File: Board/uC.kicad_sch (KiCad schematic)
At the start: 27 parts, among them U3 MP6612, U4 STM32F030K6Tx

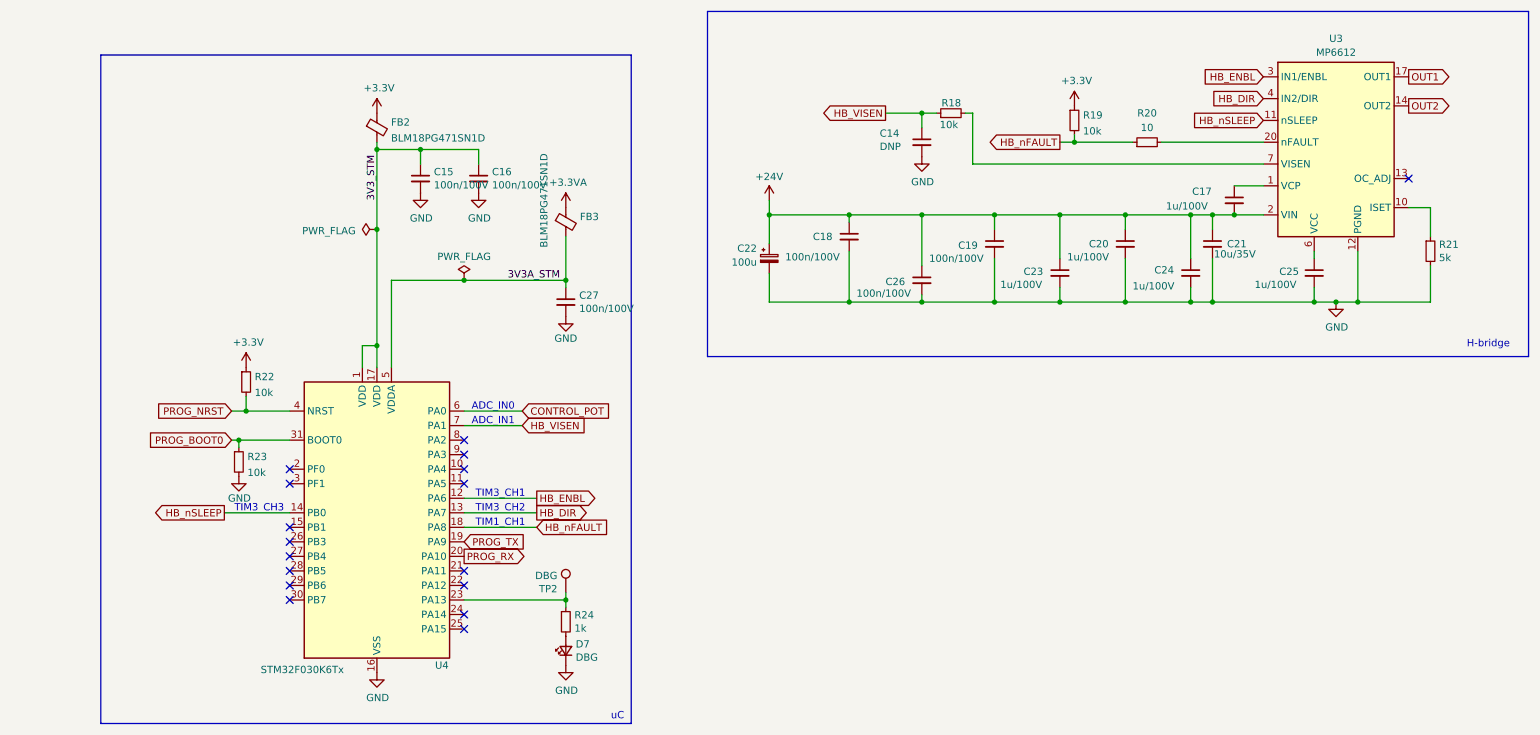
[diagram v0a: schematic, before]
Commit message: WIP on routing
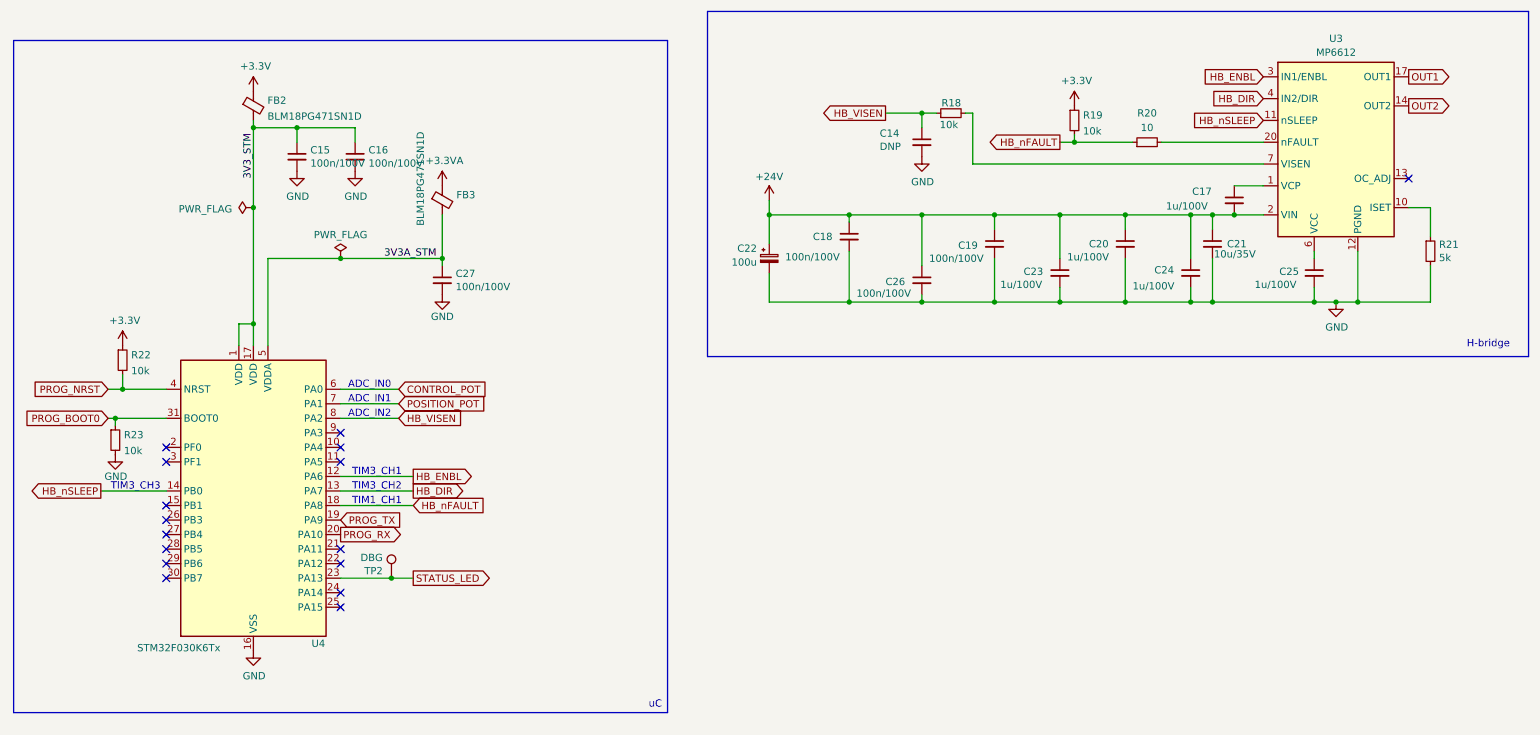
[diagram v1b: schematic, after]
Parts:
- removed D7: DBG, LED_SMD:LED_0603_1608Metric, symbol Device:LED_Small
- removed R24: 1k, Resistor_SMD:R_0603_1608Metric_Pad0.98x0.95mm_HandSolder, symbol Device:R_Small
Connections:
- net HB_VISEN: now also U4.8 (PA2); no longer U4.7 (PA1)
- net STATUS_LED: now reaches TP2.1, U4.23 (PA13)
- new net POSITION_POT: U4.7 (PA1)
- no-connect marks 17 -> 16
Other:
- note added: "ADC_IN2"
- moved on the sheet: C15, C16, C27, FB2, FB3, R22, R23, TP2, U4
